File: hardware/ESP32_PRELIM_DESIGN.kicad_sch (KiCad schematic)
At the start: 81 parts, among them J1 Conn_01x02_Pin, J2 Conn_01x11_Socket, J3 Conn_01x05_Pin, J4 Conn_01x05_Pin, J5 USB_C_Receptacle_USB2.0_16P, M1 Motor_DC, Q1 2N7002, SW1 SW_Push, SW2 SW_Push, SW3 SW_Push, U1 DRV2605LDGS, U2 ESP32-S3-WROOM-1, U3 MAX98357A, U4 MAX17048G_T10, U5 USBLC6-2SC6, U6 TPS63020DSJR, U7 BQ24075RGT

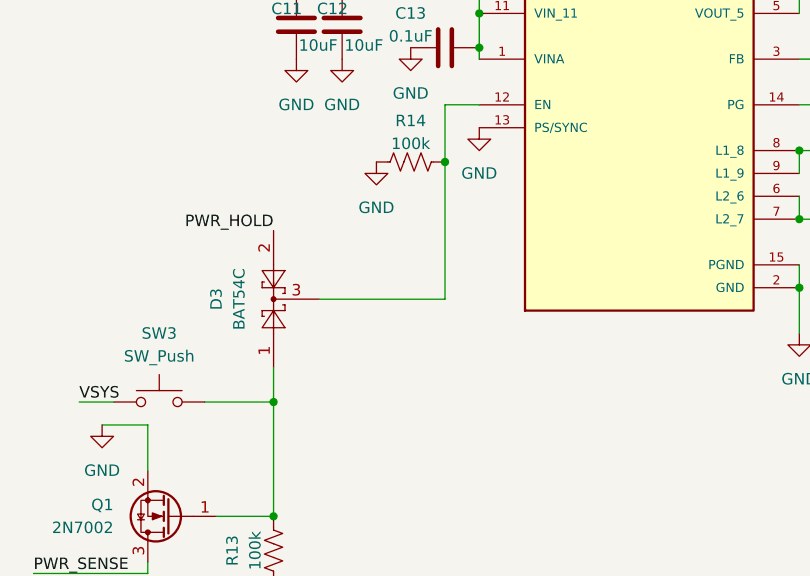
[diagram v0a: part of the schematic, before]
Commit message: final check before fabrication
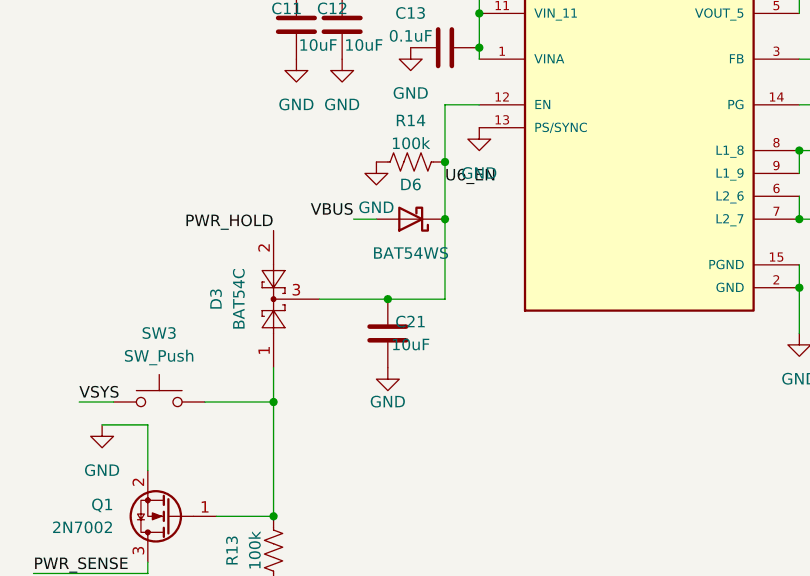
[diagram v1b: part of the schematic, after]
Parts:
- added C21: 10uF, Capacitor_SMD:C_0805_2012Metric_Pad1.18x1.45mm_HandSolder, symbol Device:C
- added D6: BAT54WS, Diode_SMD:D_SOD-323_HandSoldering, symbol Device:D_Schottky
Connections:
- net GND: now also C21.2
- net VBUS: now also D6.2 (A)
- net U6_EN: now reaches D3.3, R14.2, U6.12 (EN)
- net U6_EN: now also C21.1, D6.1 (K)
